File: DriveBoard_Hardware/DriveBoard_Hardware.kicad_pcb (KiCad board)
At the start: 2 copper layers, 61 x 99.3 mm, 51 parts, among them SW1 SW_Push, SW2 SW_Push, SW3 SW_Push, SW4 SW_Push, SW5 SW_Push, SW6 SW_Push, SW7 SW_SPDT, U1 MAX_3232, U2 MAX_3232, U3 OKI, U4 TM4C129E_Launchpad

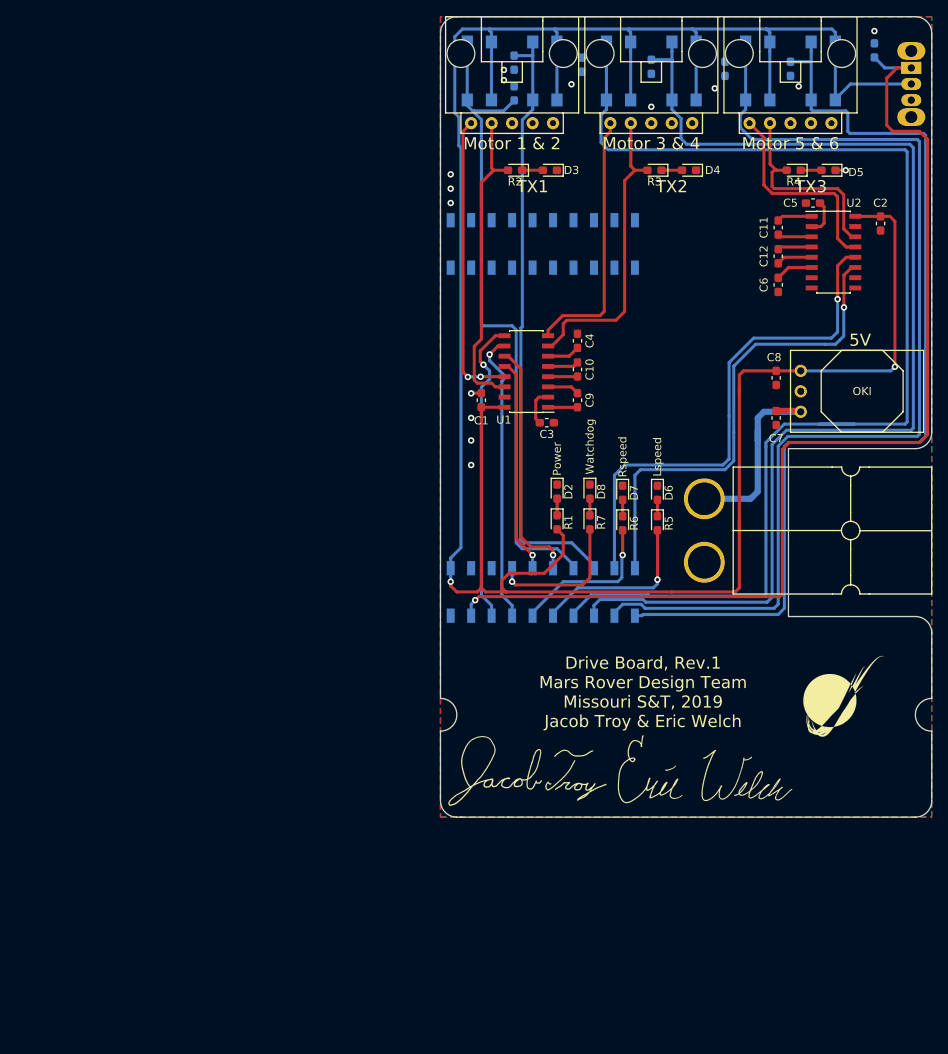
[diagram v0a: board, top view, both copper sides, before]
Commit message: Created rev 2
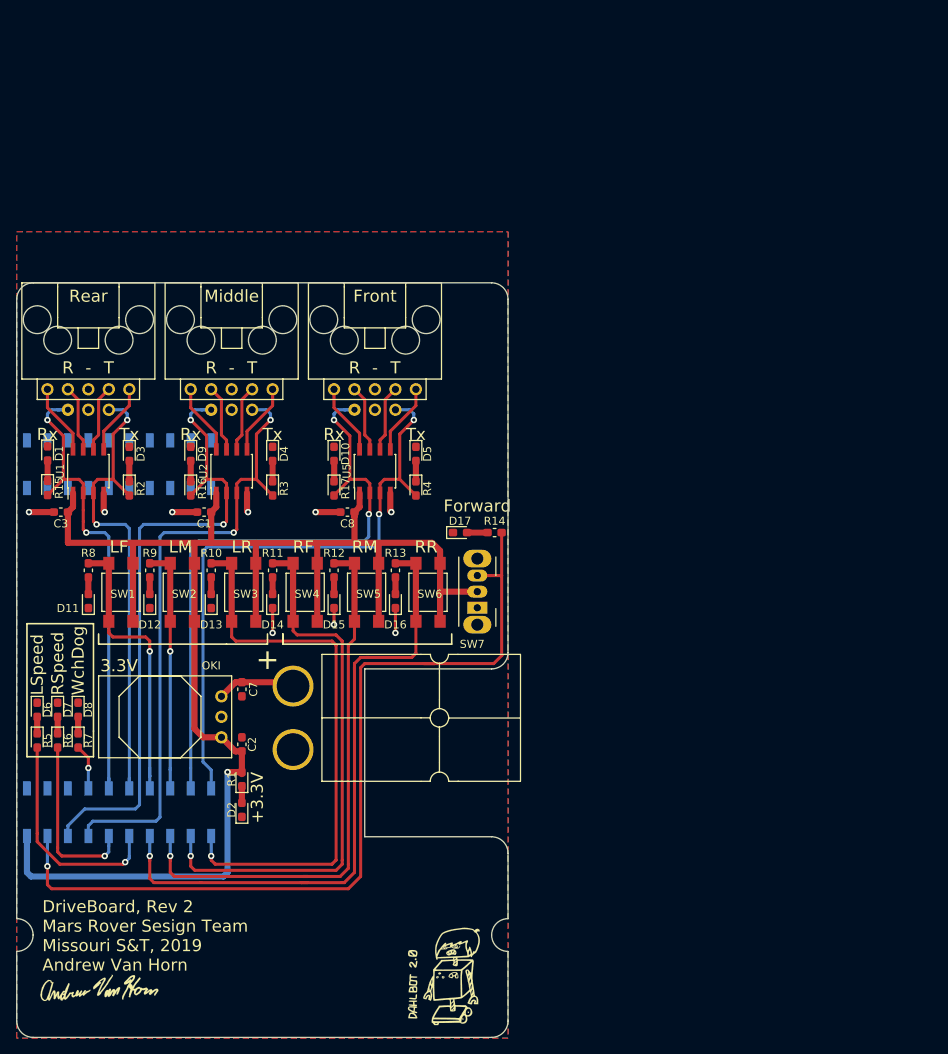
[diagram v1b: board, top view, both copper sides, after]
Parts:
- removed C10, C11, C12, C9: .1uF, Capacitor_SMD:C_0603_1608Metric_Pad1.05x0.95mm_HandSolder
- removed C4, C5, C6: 10uF, Capacitor_SMD:C_0603_1608Metric_Pad1.05x0.95mm_HandSolder
- removed the G*** at (172.5, 120.1)
- removed the G*** at (155.2, 130.0)
- removed the G*** at (132.3, 129.8)
- added Conn5: Molex_SL_03, MRDT_Connectors:MOLEX_SL_03_Horizontal, B.Cu at (78.7, 84.6)
- added Conn6: Molex_SL_03, MRDT_Connectors:MOLEX_SL_03_Horizontal, B.Cu at (96.5, 84.6)
- added Conn7: Molex_SL_03, MRDT_Connectors:MOLEX_SL_03_Horizontal, B.Cu at (114.3, 84.6)
- added D1: LED, LED_SMD:LED_0603_1608Metric_Pad1.05x0.95mm_HandSolder, F.Cu at (73.7, 90.0)
- added D10: LED, LED_SMD:LED_0603_1608Metric_Pad1.05x0.95mm_HandSolder, F.Cu at (109.2, 90.1)
- added D11: LED, LED_SMD:LED_0603_1608Metric_Pad1.05x0.95mm_HandSolder, F.Cu at (78.7, 108.3)
- added D12: LED, LED_SMD:LED_0603_1608Metric_Pad1.05x0.95mm_HandSolder, F.Cu at (86.4, 108.3)
- added D13: LED, LED_SMD:LED_0603_1608Metric_Pad1.05x0.95mm_HandSolder, F.Cu at (94.0, 108.3)
- added D14: LED, LED_SMD:LED_0603_1608Metric_Pad1.05x0.95mm_HandSolder, F.Cu at (101.6, 108.3)
- added D15: LED, LED_SMD:LED_0603_1608Metric_Pad1.05x0.95mm_HandSolder, F.Cu at (109.2, 108.3)
- added D16: LED, LED_SMD:LED_0603_1608Metric_Pad1.05x0.95mm_HandSolder, F.Cu at (116.8, 108.3)
- added D17: LED, LED_SMD:LED_0603_1608Metric_Pad1.05x0.95mm_HandSolder, F.Cu at (124.9, 99.8)
- added D9: LED, LED_SMD:LED_0603_1608Metric_Pad1.05x0.95mm_HandSolder, F.Cu at (91.4, 90.1)
- added G***: LOGO, MRDT_Silkscreens:z_sig_Andrew_Van_Horn_Sig_15mm, F.Cu at (80.0, 156.2)
- added G***: LOGO, MRDT_Silkscreens:2_Dahlbot_2.0, F.Cu at (122.6, 154.9)
- added R15: 500, LED_SMD:LED_0603_1608Metric_Pad1.05x0.95mm_HandSolder, F.Cu at (73.7, 94.3)
- added R16: 500, LED_SMD:LED_0603_1608Metric_Pad1.05x0.95mm_HandSolder, F.Cu at (91.4, 94.3)
- added R17: 500, LED_SMD:LED_0603_1608Metric_Pad1.05x0.95mm_HandSolder, F.Cu at (109.2, 94.3)
- added U5: MAX3077E, Package_SO:SOIC-8_3.9x4.9mm_P1.27mm, F.Cu at (114.3, 92.2)
- C1, C2: value .1uF -> 10u
- C3: value 10uF -> 10u
- R10, R11, R12, R13, R14, R8, R9, SW1, SW2, SW3, SW4, SW5, SW6, SW7: moved to F.Cu
- U1, U2: value MAX_3232 -> MAX3077E; footprint Package_SO:SOIC-16_3.9x9.9mm_P1.27mm -> Package_SO:SOIC-8_3.9x4.9mm_P1.27mm
- moved C2 102.3 mm to (97.8, 126.1)
- moved SW7 85.9 mm to (127.0, 109.2), turned to 90 degrees
- moved R5 81.5 mm to (72.4, 125.6)
- moved D6 81.5 mm to (72.4, 121.8)
- moved SW6 81.2 mm to (120.9, 107.2), turned to 270 degrees
- moved SW5 80.9 mm to (113.3, 107.2), turned to 270 degrees
- moved SW4 80.0 mm to (105.6, 107.2), turned to 270 degrees
- moved SW3 79.7 mm to (98.0, 107.2), turned to 270 degrees
- moved U2 79.5 mm to (96.5, 92.2), turned to 90 degrees
- moved R8 79.3 mm to (78.7, 104.5), turned to 90 degrees
- moved R13 79.2 mm to (116.8, 104.5)
- moved R12 78.9 mm to (109.2, 104.5)
- moved SW2 78.8 mm to (90.4, 107.2), turned to 270 degrees
- moved SW1 78.5 mm to (82.8, 107.2), turned to 270 degrees
- moved R11 78.2 mm to (101.6, 104.5)
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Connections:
- C1 pad 1: GND -> +3V3
- C1 pad 2: +5V -> GND
- C2 pad 1: GND -> +3V3
- C2 pad 2: +5V -> GND
- C3 pad 1: GND -> +3V3
- C3 pad 2: Net-(C3-Pad2) -> GND
- C8 pad 1: +5V -> +3V3
- Conn2 pad 1: RX_1_SL -> A1
- Conn2 pad 2: TX_1_SL -> B1
- Conn2 pad 3: Net-(Conn2-Pad3) -> GND
- Conn2 pad 4: Net-(Conn2-Pad4) -> Z1
- Conn2 pad 5: GND -> Y1
- Conn3 pad 1: RX_2_SL -> A2
- Conn3 pad 2: TX_2_SL -> B2
- Conn3 pad 3: Net-(Conn3-Pad3) -> GND
- Conn3 pad 4: Net-(Conn3-Pad4) -> Z2
- Conn3 pad 5: GND -> Y2
- Conn4 pad 1: RX_3_SL -> A3
- Conn4 pad 2: TX_3_SL -> B3
- Conn4 pad 3: Net-(Conn4-Pad3) -> GND
- Conn4 pad 4: Net-(Conn4-Pad4) -> Z3
- Conn4 pad 5: GND -> Y3
- R1 pad 2: +5V -> +3V3
- R10 pad 1: GND -> Net-(D13-Pad2)
- R11 pad 1: GND -> Net-(D14-Pad2)
- R12 pad 1: GND -> Net-(D15-Pad2)
- R13 pad 1: GND -> Net-(D16-Pad2)
- R14 pad 1: GND -> Net-(D17-Pad2)
- R2 pad 2: TX_1_SL -> TX_1
- R3 pad 2: TX_2_SL -> TX_2
- R4 pad 2: TX_3_SL -> TX_3
- R8 pad 1: GND -> Net-(D11-Pad2)
- R9 pad 1: GND -> Net-(D12-Pad2)
- SW1 pad 1: +5V -> +3V3
- SW2 pad 1: +5V -> +3V3
- SW3 pad 1: +5V -> +3V3
- SW4 pad 1: +5V -> +3V3
- SW5 pad 1: +5V -> +3V3
- SW6 pad 1: +5V -> +3V3
- SW7 pad 1: DIRECTION_SW -> Net-(SW7-Pad1)
- SW7 pad 2: +5V -> +3V3
- SW7 pad 3: (no net) -> DIRECTION_SW
- U1 pad 1: Net-(C9-Pad2) -> +3V3
- U1 pad 2: Net-(C3-Pad2) -> RX_1
- U1 pad 3: Net-(C9-Pad1) -> TX_1
- U1 pad 4: Net-(C10-Pad2) -> GND
- U1 pad 5: Net-(C10-Pad1) -> Y1
- U1 pad 6: Net-(C4-Pad2) -> Z1
- U1 pad 7: TX_2_SL -> B1
- U1 pad 8: RX_2_SL -> A1
- U2 pad 1: Net-(C11-Pad2) -> +3V3
- U2 pad 2: Net-(C5-Pad2) -> RX_2
- U2 pad 3: Net-(C11-Pad1) -> TX_2
- U2 pad 4: Net-(C12-Pad2) -> GND
- U2 pad 5: Net-(C12-Pad1) -> Y2
- U2 pad 6: Net-(C6-Pad2) -> Z2
- U2 pad 7: (no net) -> B2
- U2 pad 8: (no net) -> A2
- U3 pad 3: +5V -> +3V3
- U4 pad +3V3': (no net) -> +3V3
- U4 pad +5V': +5V -> Net-(U4-Pad+5V')
- U4 pad PA4: RX_3_IC -> RX_3
- U4 pad PA5: TX_3_IC -> TX_3
- U4 pad PK0: RX_1_IC -> RX_1
- U4 pad PK1: TX_1_IC -> TX_1
- U4 pad PN4: M6_SW -> M3_SW
- U4 pad PN5: M5_SW -> M4_SW
- U4 pad PP0: RX_2_IC -> RX_2
- U4 pad PP1: TX_2_IC -> TX_2
- U4 pad PP4: M4_SW -> M5_SW
- U4 pad PQ0: M3_SW -> M6_SW
- U4 pad Rese': (no net) -> Net-(U4-PadRese')
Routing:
- net +5V: track 327.9 -> 0.00 mm, vias 2 -> 0
- net +3V3: track 0.00 -> 196.4 mm, vias 0 -> 1
- net M3_SW: track 154.9 -> 70.7 mm, vias 0 -> 1
- net RX_2: track 0.00 -> 79.8 mm, vias 0 -> 2
- net TX_2: track 0.00 -> 77.8 mm, vias 0 -> 2
- net RX_3: track 0.00 -> 77.5 mm, vias 0 -> 2
- net TX_3: track 0.00 -> 76.4 mm, vias 0 -> 2
- net M4_SW: track 140.5 -> 68.4 mm, vias 0 -> 1
- net RX_3_IC: track 64.5 -> 0.00 mm, vias 1 -> 0
- net M5_SW: track 132.1 -> 68.5 mm, vias 0 -> 1
- net TX_3_IC: track 60.8 -> 0.00 mm, vias 1 -> 0
- net RX_1: track 0.00 -> 60.2 mm, vias 0 -> 2
- net TX_1: track 0.00 -> 59.9 mm, vias 0 -> 2
- net M1_SW: track 81.0 -> 36.0 mm, vias 0 -> 1
- net M2_SW: track 75.4 -> 31.2 mm, vias 0 -> 1
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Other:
- board size 61 x 99.3 mm -> 61 x 93.6 mm
- board text added: "+"
- board text added: "+3.3V"
- board text added: "3 RS-485 3 UART"
- board text added: "3.3V"
- board text added: "A"
- board text added: "B"
- board text added: "DriveBoard, Rev 2 Mars Rover Sesign Team Missouri S&T, 2019 Andrew Van Horn"
- board text added: "Forward"
- board text added: "Front"
- board text added: "LF"
- board text added: "LM"
- board text added: "LR"
- board text added: "LSpeed"
- board text added: "Middle"
- board text added: "R"
- board text added: "RF"
- board text added: "RM"
- board text added: "RR"
- board text added: "RSpeed"
- board text added: "Rear"
- board text added: "T"
- board text added: "WchDog"
- board text added: "Y"
- board text added: "Z"
- board text removed: "5V"
- board text removed: "Drive Board, Rev.1 Mars Rover Design Team Missouri S&T, 2019 Jacob Troy & Eric Welch"
- board text removed: "FWD"
- board text removed: "Lspeed"
- board text removed: "M1"
- board text removed: "M2"
- board text removed: "M3"
- board text removed: "M4"
- board text removed: "M5"
- board text removed: "M6"
- board text removed: "Motor 1 & 2"
- board text removed: "Motor 3 & 4"
- board text removed: "Motor 5 & 6"
- board text removed: "Power"
- board text removed: "REV"
- board text removed: "Rspeed"
- board text removed: "TX1"
- board text removed: "TX2"
- board text removed: "TX3"
- board text removed: "Watchdog"
